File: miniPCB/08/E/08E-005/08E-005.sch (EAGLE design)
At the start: 57 parts, among them U1 OPAMP_QUADTHD

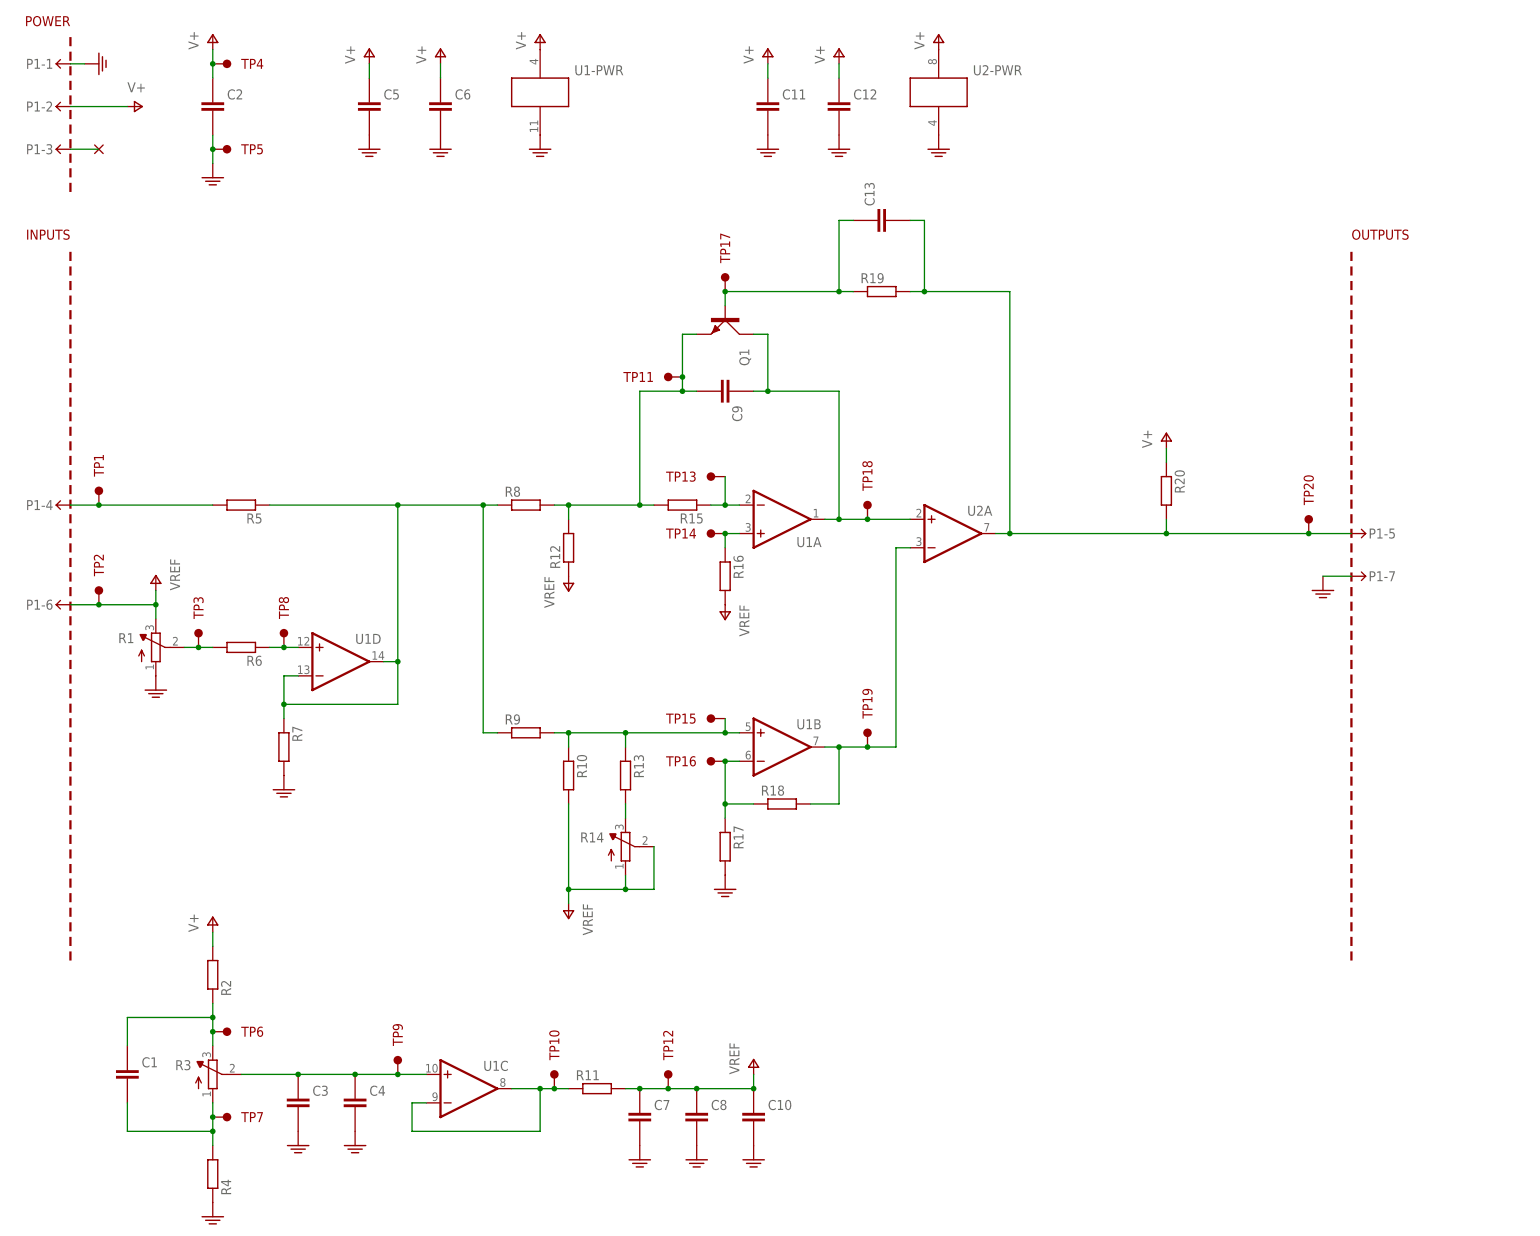
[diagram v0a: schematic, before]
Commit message: Attempting to fix my Git merge error.
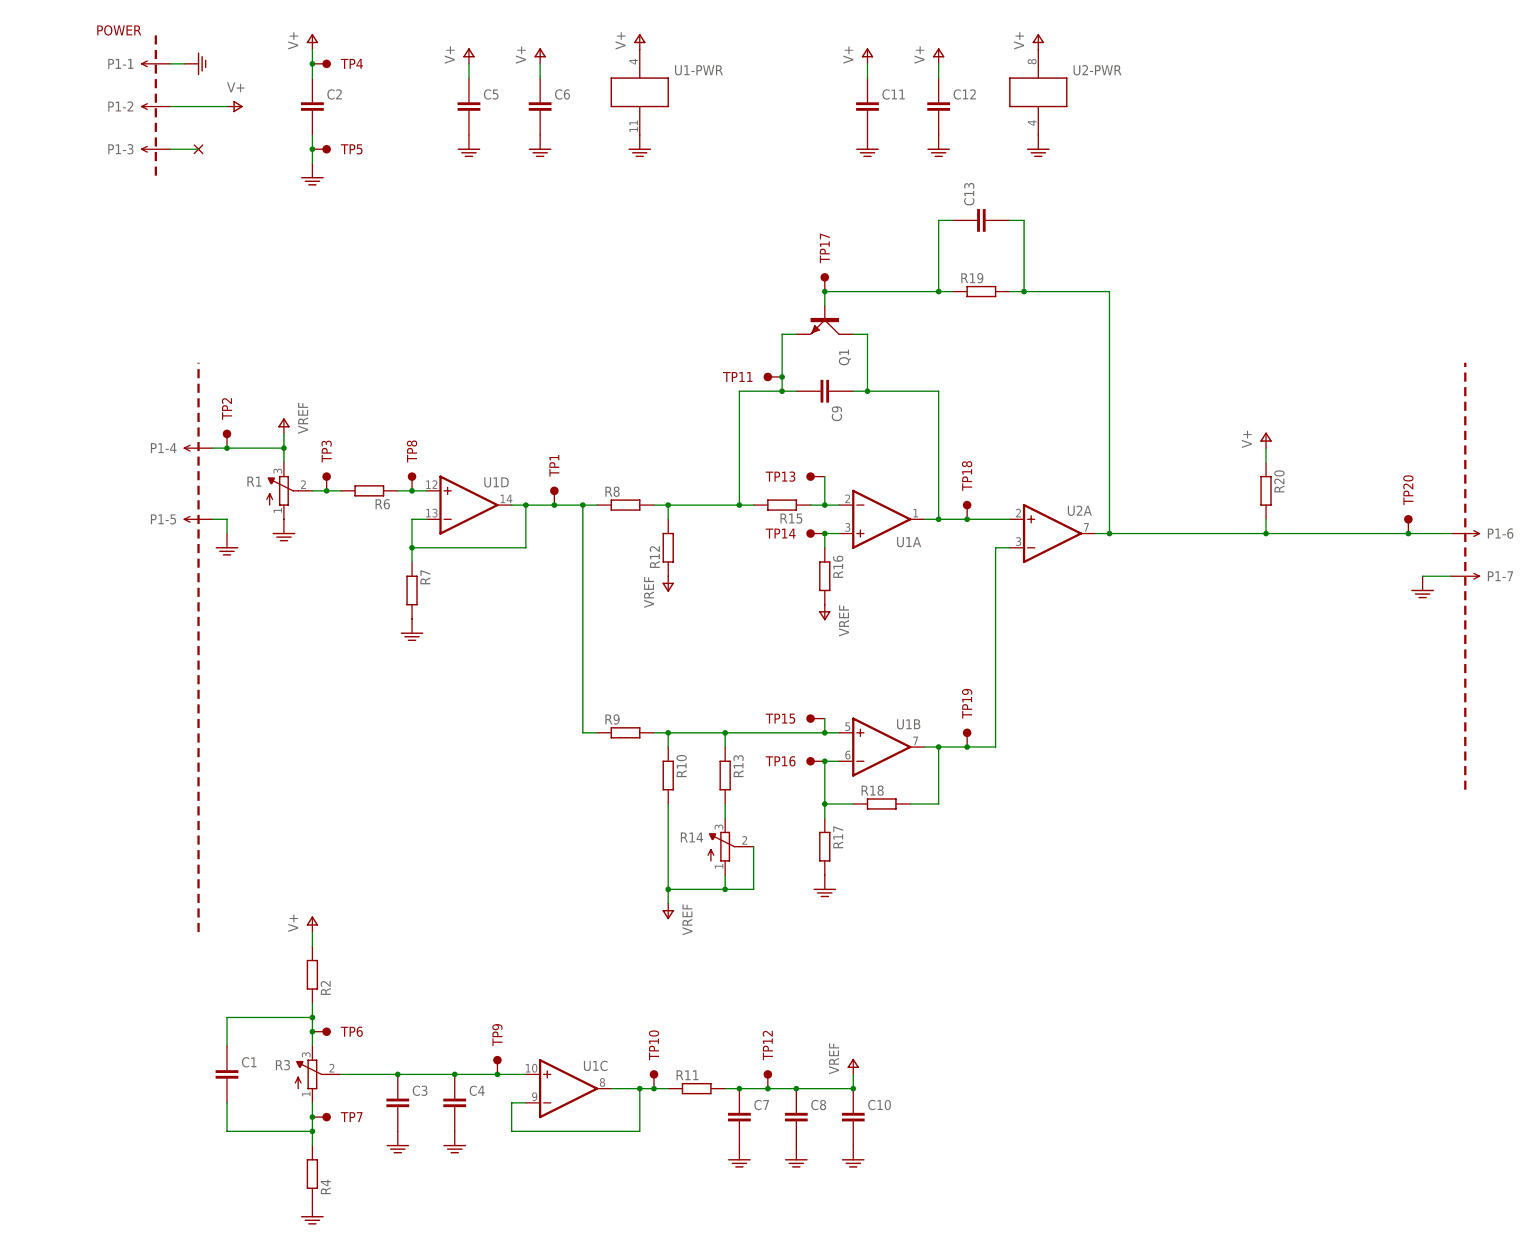
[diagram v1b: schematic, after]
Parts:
- removed P1-: (no value), minipcb:MINIPCB_7P50X100
- removed R5: (no value), minipcb:RESISTOR10MM
- added P1: (no value), minipcb:MINIPCB_7P
- added PCB1: POWER, minipcb:MINIPCB_0P50X75
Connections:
- removed net N$1: P1-4.1, R5.2, TP1.1
- net GND: now also P1-1.1, P1-5.1, P1-7.1; no longer P1-1.1, P1-7.1
- net N$4: now also TP1.1; no longer R5.1
- net N$6: now also P1-6.1; no longer P1-5.1
- net NC: now also P1-3.1; no longer P1-3.1
- net V+: now also P1-2.1; no longer P1-2.1
- net VREF: now also P1-4.1; no longer P1-6.1
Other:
- moved on the sheet: C1, C10, C11, C12, C13, C2, C3, C4, C5, C6, C7, C8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

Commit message: Attempting to fix my Git merge error.
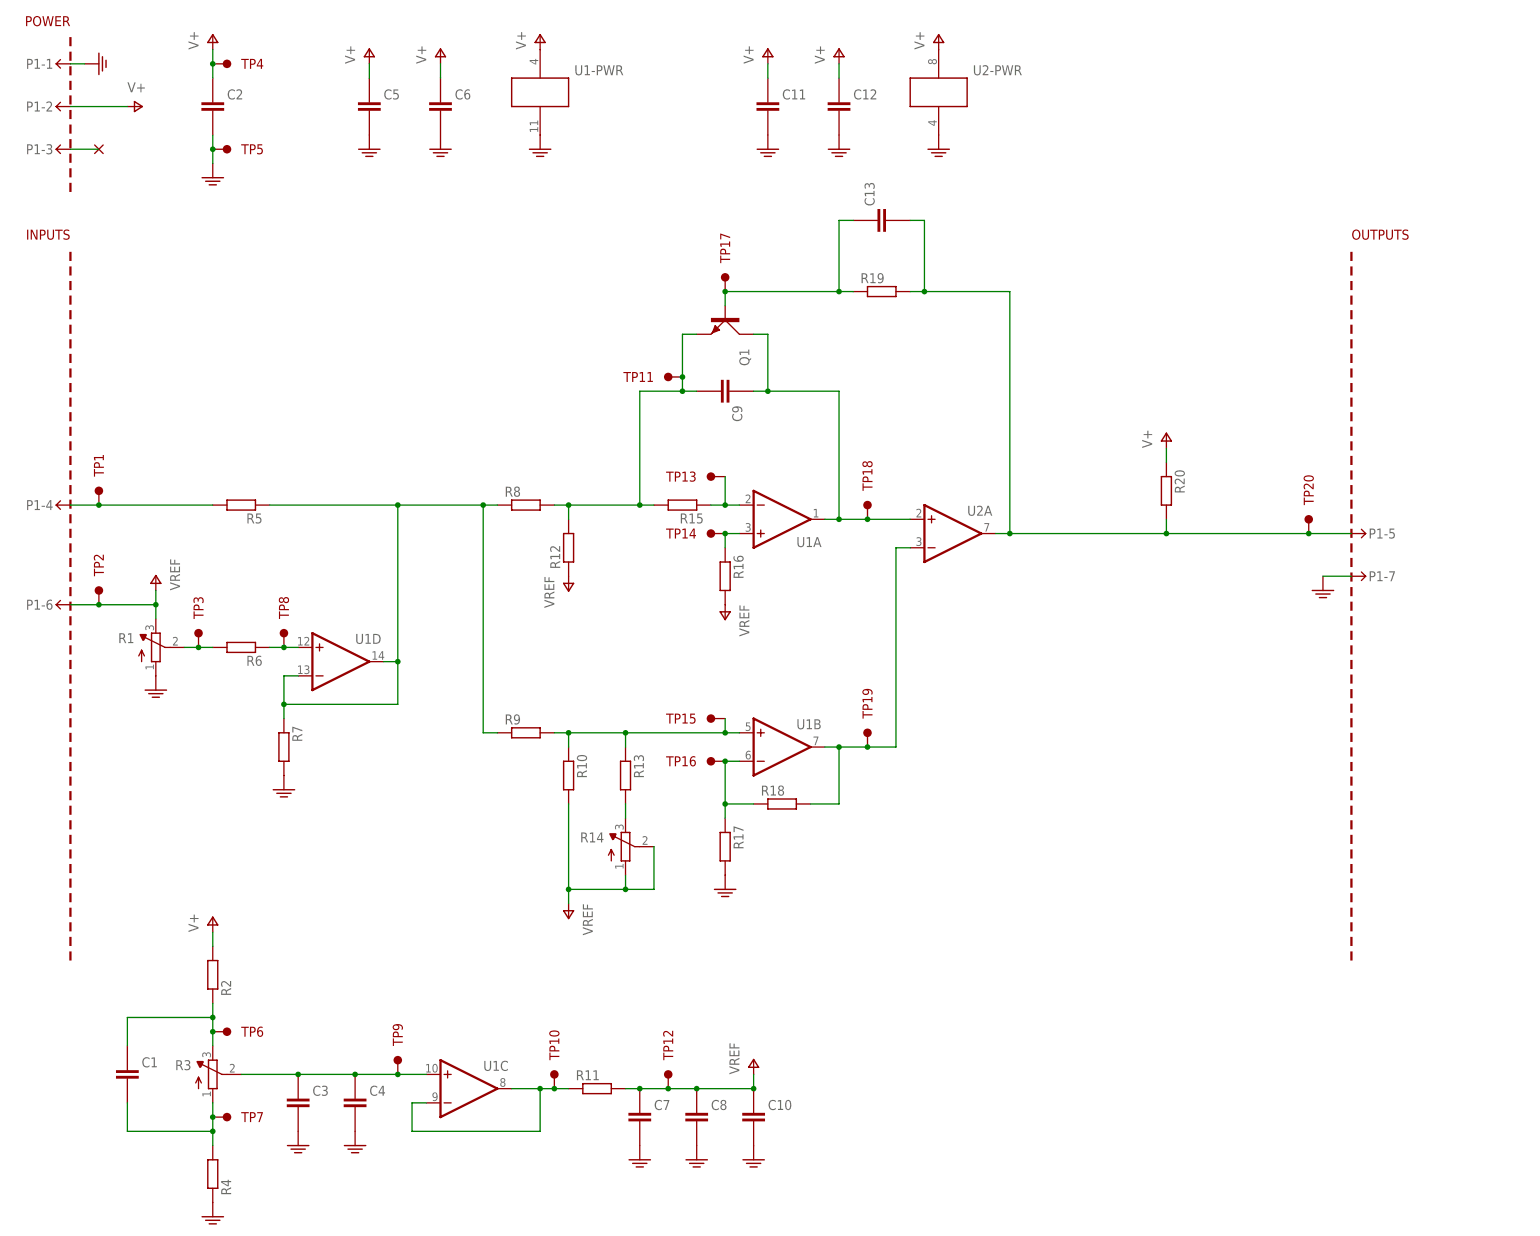
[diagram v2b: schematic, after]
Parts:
- removed P1: (no value), minipcb:MINIPCB_7P
- removed PCB1: POWER, minipcb:MINIPCB_0P50X75
- added P1-: (no value), minipcb:MINIPCB_7P50X100
- added R5: (no value), minipcb:RESISTOR10MM
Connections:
- new net N$1: P1-4.1, R5.2, TP1.1
- net GND: now also P1-1.1, P1-7.1; no longer P1-1.1, P1-5.1, P1-7.1
- net N$4: now also R5.1; no longer TP1.1
- net N$6: now also P1-5.1; no longer P1-6.1
- net NC: now also P1-3.1; no longer P1-3.1
- net V+: now also P1-2.1; no longer P1-2.1
- net VREF: now also P1-6.1; no longer P1-4.1
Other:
- moved on the sheet: C1, C10, C11, C12, C13, C2, C3, C4, C5, C6, C7, C8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
